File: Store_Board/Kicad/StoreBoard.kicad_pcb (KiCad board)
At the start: 2 copper layers, 230 x 78 mm, 36 parts, among them J1 Conn_01x10, J2 Conn_01x10, J3 Conn_01x10, J4 Conn_01x10, U1 HM62256BLP, U2 74HCT574, U3 74HCT574, U4 74HCT04, U417 74LS00, U418 74LS00, U419 74LS08, U420 74HC04, U421 74LS112, U422 SN74LS74, U423 74LS10, U424 74LS32

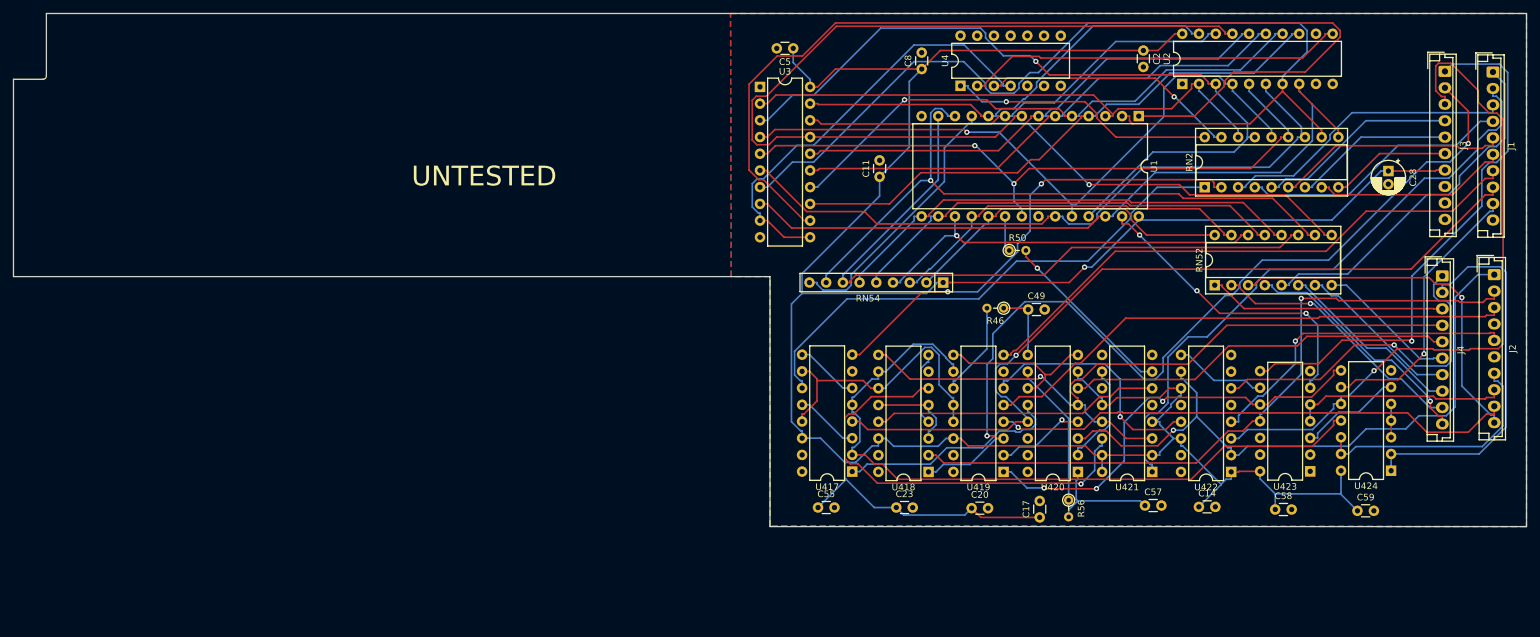
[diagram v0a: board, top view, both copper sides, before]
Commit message: Ready for testing, I think
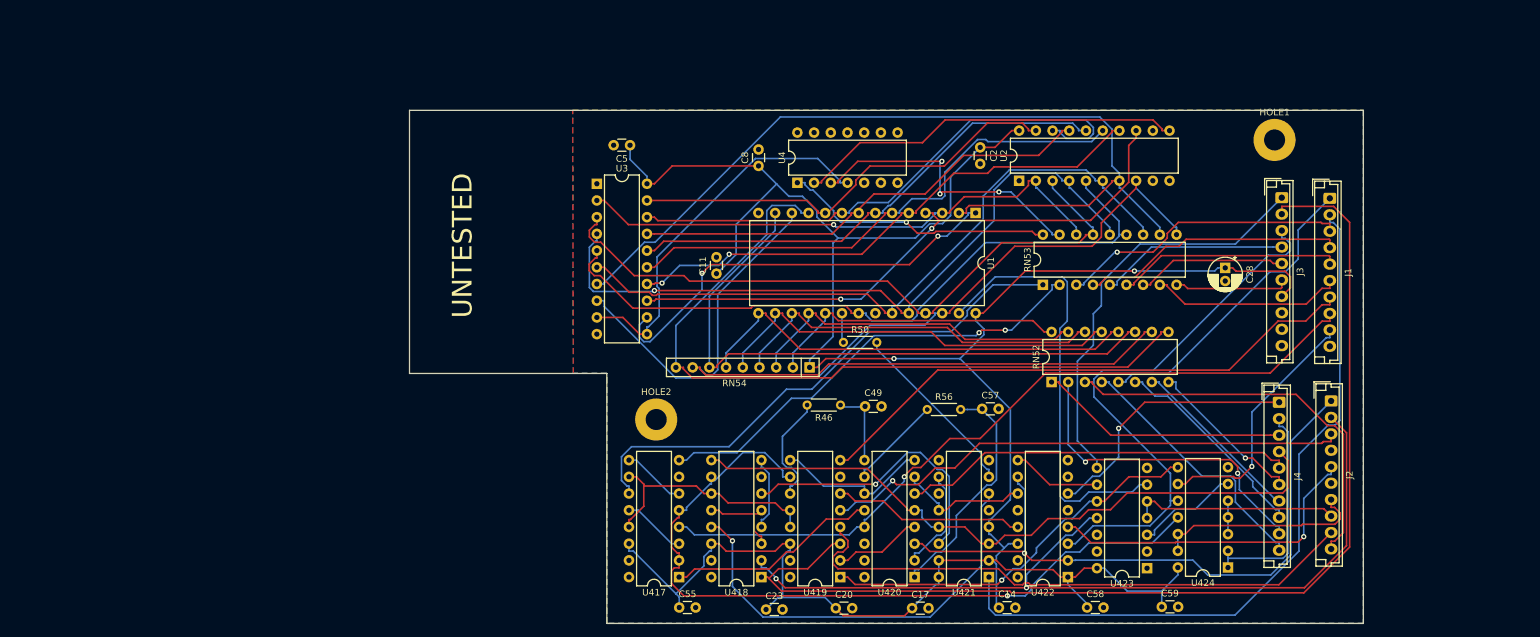
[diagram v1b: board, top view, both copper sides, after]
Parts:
- removed RN2: 33, Package_DIP:DIP-18_W7.62mm_Socket
- added HOLE1: HOLE, MountingHole:MountingHole_3.2mm_M3_Pad, F.Cu at (236.7, 59.2)
- added HOLE2: HOLE, MountingHole:MountingHole_3.2mm_M3_Pad, F.Cu at (142.7, 101.7)
- added RN53: 33, Package_DIP:DIP-18_W7.62mm, F.Cu at (201.5, 81.2)
- R46, R50, R56: footprint Resistor_THT:R_Axial_DIN0204_L3.6mm_D1.6mm_P2.54mm_Vertical -> Resistor_THT:R_Axial_DIN0204_L3.6mm_D1.6mm_P5.08mm_Horizontal
- RN52: footprint Package_DIP:DIP-16_W7.62mm_Socket -> Package_DIP:DIP-16_W7.62mm
- moved C14 34.0 mm to (194.8, 130.3)
- moved C59 33.1 mm to (219.6, 130.2)
- moved C58 32.2 mm to (208.2, 130.3)
- moved J2 31.4 mm to (245.3, 98.9)
- moved J3 31.4 mm to (237.8, 68.0)
- moved J1 31.4 mm to (245.1, 68.1)
- moved J4 31.4 mm to (237.4, 99.1)
- moved U417 30.8 mm to (146.2, 125.7)
- moved U418 30.0 mm to (158.7, 125.7)
- moved U420 29.5 mm to (182.0, 125.7)
- moved U419 29.5 mm to (170.7, 125.7)
- moved U421 29.5 mm to (193.3, 125.7)
- moved U422 29.5 mm to (205.3, 125.7)
- moved C49 28.8 mm to (174.4, 99.7)
- moved C5 28.8 mm to (138.7, 60.0)
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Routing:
- net /RAS_A14: track 156.9 -> 64.6 mm, vias 0 -> 2
- net /RAS_A2: track 127.6 -> 71.6 mm
- net /TVAD: track 137.7 -> 168.2 mm, vias 2 -> 0
- net /1\4: track 105.9 -> 130.8 mm, vias 1 -> 2
- net /~{RD}: track 57.6 -> 33.3 mm
- net Net-(U421B-~{R}): track 66.7 -> 43.5 mm
- net Net-(U421A-~{Q}): track 43.7 -> 65.6 mm, vias 0 -> 1
- net VCC: track 424.0 -> 403.8 mm, vias 1 -> 2
- net /~{TVCLK}: track 83.1 -> 63.7 mm, vias 1 -> 0
- net /1\2: track 104.3 -> 85.0 mm, vias 1 -> 0
- net Net-(U1-~{WE}): track 47.4 -> 66.7 mm, vias 3 -> 0
- net /ZCK: track 93.2 -> 111.6 mm
- net /A1: track 119.7 -> 101.3 mm, vias 1 -> 0
- net Net-(C57-Pad1): track 18.1 -> 36.1 mm
- net /RAS_A1: track 68.0 -> 83.3 mm
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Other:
- board size 230 x 78 mm -> 145 x 78 mm
